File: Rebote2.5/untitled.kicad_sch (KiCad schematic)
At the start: 14 parts, among them J1 V+ GND, J2 IN, J3 OUT, J4 V+ GND, SW1 SW_3PDT

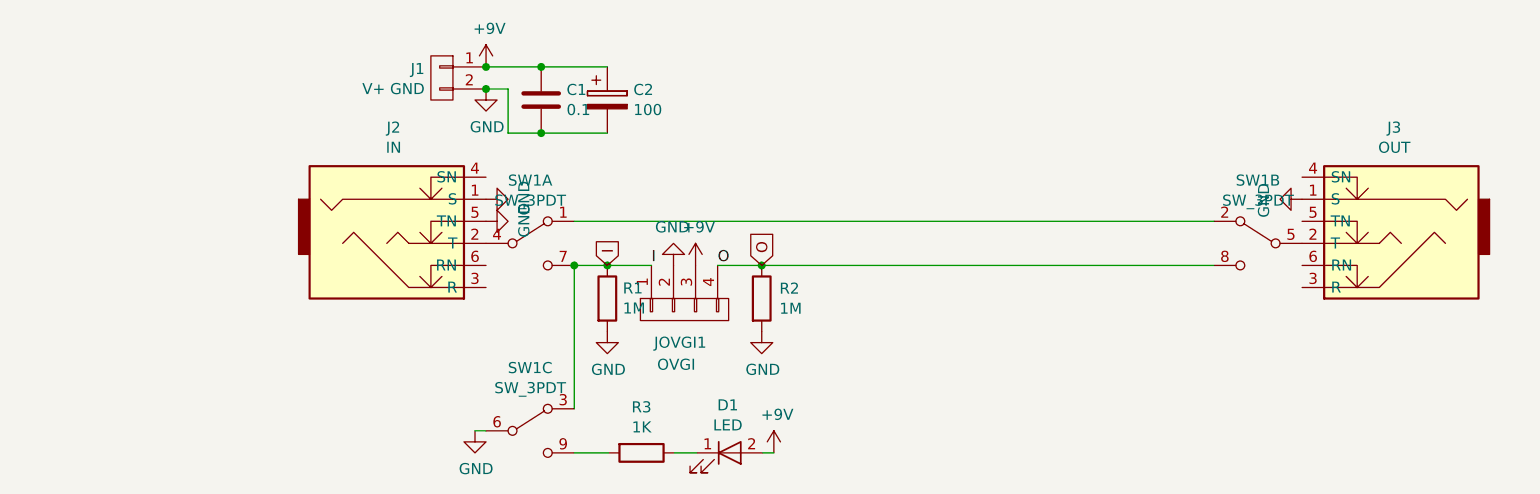
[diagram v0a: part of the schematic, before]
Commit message: WIP
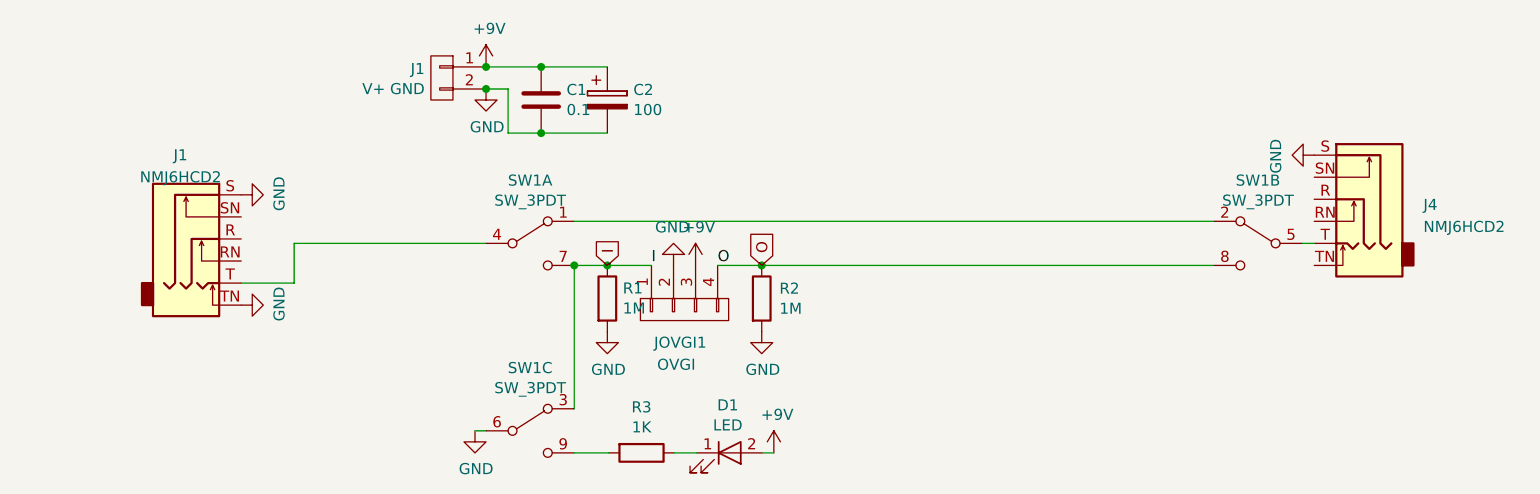
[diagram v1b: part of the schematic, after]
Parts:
- removed J2: IN, Connectors:NMJ6HCD2, symbol 1590B-rescue:JACK_TRS_6PINS-conn
- removed J3: OUT, Connectors:NMJ6HCD2, symbol 1590B-rescue:JACK_TRS_6PINS-conn
- added J1, J4: NMJ6HCD2, Connector_Audio:Jack_6.35mm_Neutrik_NMJ6HCD2_Horizontal, symbol Connector_Audio:NMJ6HCD2
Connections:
- net GND: now also J1.S, J1.TN, J4.S
- net at SW1.5 (B): now also J4.T
- net at SW1.4 (B): now also J1.T
